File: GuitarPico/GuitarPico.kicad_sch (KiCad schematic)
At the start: 125 parts, among them J1 INPUT, J2 INPUT, J3 OUTPUT, J4 OUTPUT, J5 Barrel_Jack_Switch, J6 VGA, J8 INPUT, J9 INPUT, Q1 2N3904, Q2 2N3904, Q3 2N3904, SW1 SW_Push, SW2 SW_Push, SW3 SW_Push, SW4 SW_Push, SW5 SW_Push, U1 LM358, U2 LM358, U3 Pico, U4 LM7805_TO220, U5 TL431LP, U6 4051

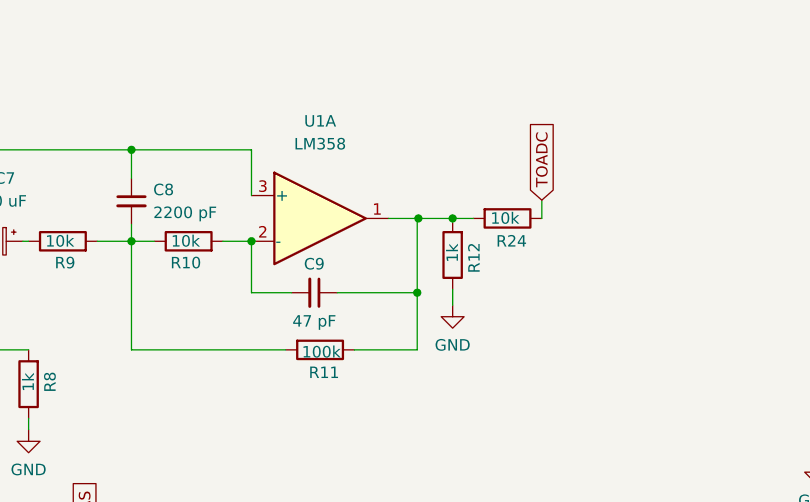
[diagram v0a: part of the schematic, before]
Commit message: First example of guitarpico project
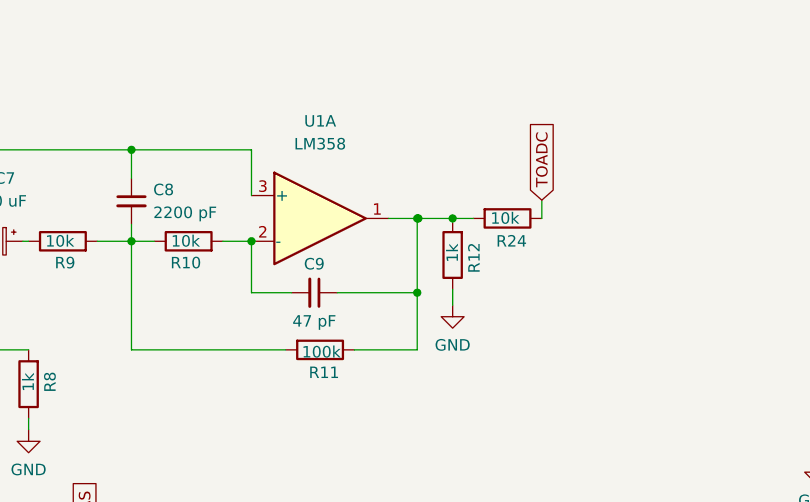
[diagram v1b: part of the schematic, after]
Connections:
- net at C9.1, R11.1, U1.1: now also R12.2, R24.2
